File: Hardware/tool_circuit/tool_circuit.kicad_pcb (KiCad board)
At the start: 2 copper layers, 65 x 56.7 mm, 31 parts, among them J1 EJ503A, J2 Conn_01x03_Female, J3 Conn_01x08_Female, J4 GPIO_CONNECTOR, SW1 1825255-1, U1 LM2576D2TR4-5G

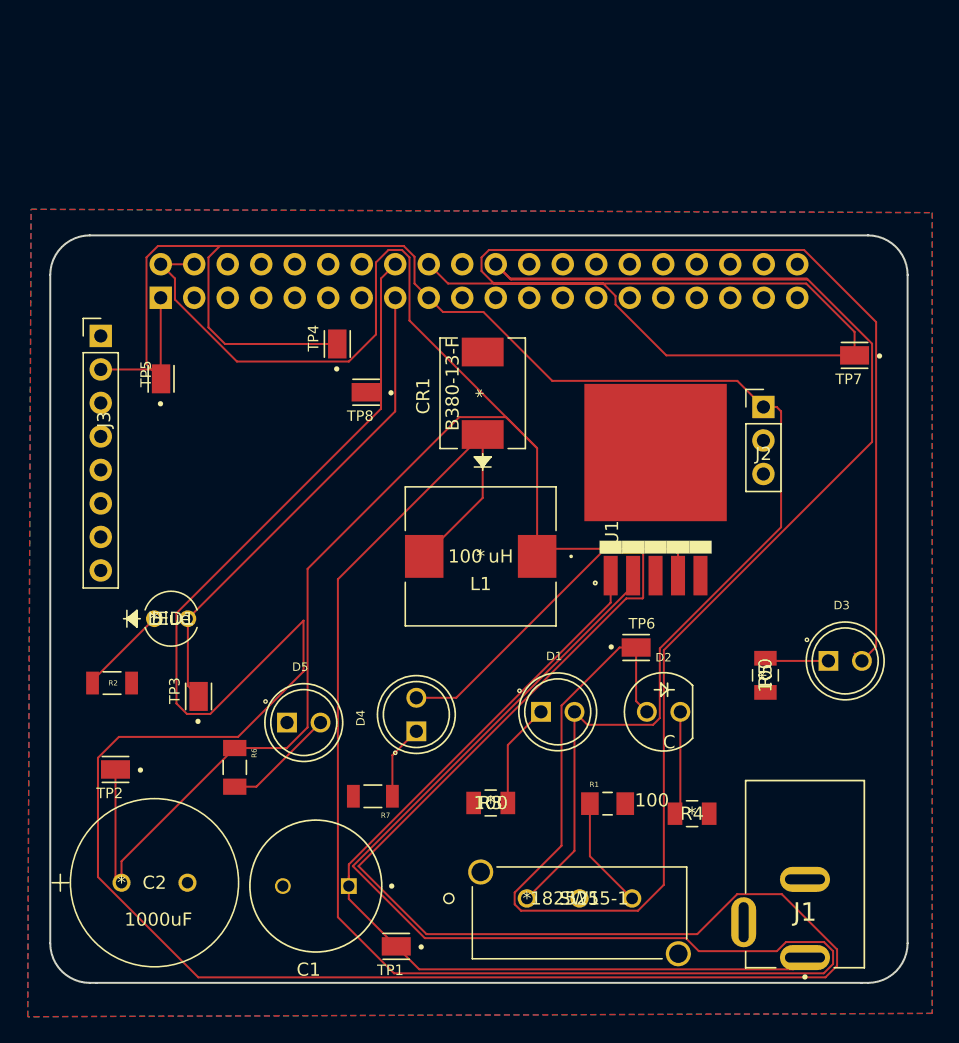
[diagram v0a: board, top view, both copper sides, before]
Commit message: pcb revisions
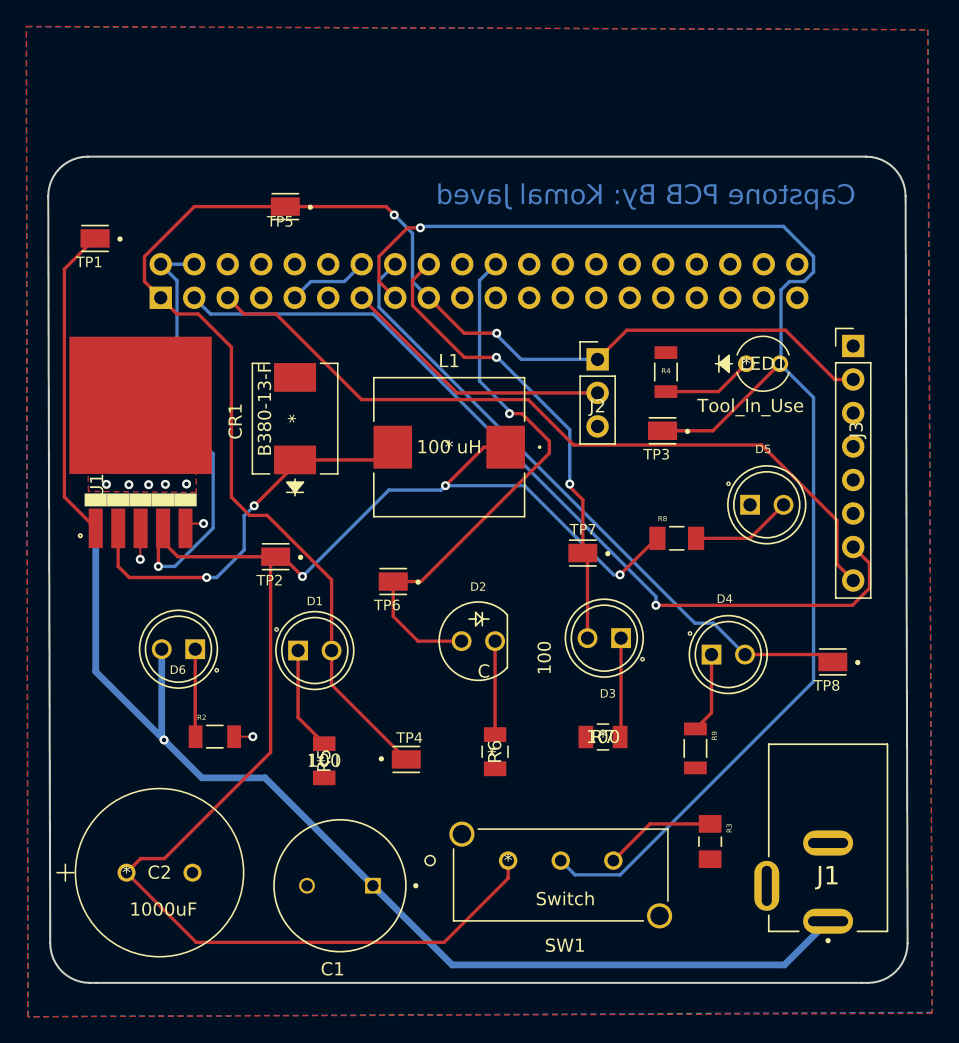
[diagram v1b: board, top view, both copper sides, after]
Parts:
- removed R1: 10k, RNCP1206FTD10K0:RESC3115X60N
- added D6: 12V, WP7113GD:LED_WP7113GD, F.Cu at (109.6, 79.7)
- added R8: 220, RMCF1206JT220R:RESC3216X70N, F.Cu at (147.4, 71.3)
- added R9: 130, AC1206FR-07130RL:RESC3116X65N, F.Cu at (148.8, 87.2)
- D1: value Green -> 3.3V
- D2: value Red -> Disable
- D3: value Green -> Enable
- D4: value Yellow -> Data_Transfer
- D5: value Green -> 5V
- J2: value Conn_01x03_Female -> Temp_Sense
- J3: value Conn_01x08_Female -> Accel.
- LED1: value Blue -> Tool_In_Use
- R2: value 42.2 -> 820; footprint RC1206FR-0742R2L:RESC3116X65N -> CRGCQ1206F820R:RESC3115X65N
- R3: value 100 -> 10k; footprint footprints:RNCP1206FTD100R -> RNCP1206FTD10K0:RESC3115X60N
- R4: value 100 -> 42.2; footprint footprints:RNCP1206FTD100R -> RC1206FR-0742R2L:RESC3116X65N
- R6: value 220 -> 100; footprint RMCF1206JT220R:RESC3216X70N -> footprints:RNCP1206FTD100R
- R7: value 130 -> 100; footprint AC1206FR-07130RL:RESC3116X65N -> footprints:RNCP1206FTD100R
- SW1: value 1825255-1 -> Switch
- TP1: value S2751-46R -> Vin
- TP2: value S2751-46R -> 5V_Reg_Vout
- TP3: value S2751-46R -> Tool_In_Use
- TP4: value S2751-46R -> 3.3V
- TP5: value S2751-46R -> GPIO1
- TP6: value S2751-46R -> Disable
- TP7: value S2751-46R -> Enable_LED
- TP8: value S2751-46R -> Data_Transfer
- moved TP1 58.3 mm to (103.3, 48.5)
- moved J3 57.1 mm to (160.8, 56.7)
- moved LED1 48.9 mm to (152.7, 58.0)
- moved TP8 40.9 mm to (159.2, 80.6)
- moved TP3 40.5 mm to (146.3, 63.1), turned to 180 degrees
- moved U1 39.2 mm to (106.7, 66.0)
- moved D5 38.8 mm to (154.2, 68.7)
- moved R5 34.1 mm to (120.7, 88.1)
- moved R4 33.5 mm to (146.6, 58.6), turned to 90 degrees
- moved TP4 31.9 mm to (126.9, 88.0), turned to 0 degrees
- moved TP7 25.5 mm to (140.3, 72.4)
- moved D4 24.1 mm to (151.3, 80.1), turned to 0 degrees
- moved TP2 20.2 mm to (117.0, 72.6)
- moved R6 19.8 mm to (133.6, 87.4)
- moved TP6 19.1 mm to (125.9, 74.5), turned to 180 degrees
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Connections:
- J2 pad 2: /Temp_Sense/GPIO27 -> GPIO27_GEN2
- J3 pad 7: /Accelerometer.sch/GPIO2 -> GPIO2_SDA1
- J3 pad 8: /Accelerometer.sch/GPIO3 -> GPIO3_SCL1
- J4 pad 13: /raspberrypi_header.sch/GPIO27 -> GPIO27_GEN2
- J4 pad 15: /raspberrypi_header.sch/GPIO22_GEN3 -> GPIO22_GEN3
- J4 pad 3: /raspberrypi_header.sch/GPIO2 -> GPIO2_SDA1
- J4 pad 5: /raspberrypi_header.sch/GPIO3 -> GPIO3_SCL1
- LED1 pad 2: /raspberrypi_header.sch/GPIO22_GEN3 -> GPIO22_GEN3
- R2 pad 1: Net-(LED1-Pad1) -> Net-(D6-PadC)
- R3 pad 1: Net-(D1-PadC) -> Net-(R3-Pad1)
- R4 pad 1: Net-(D2-Pad1) -> Net-(LED1-Pad1)
- R5 pad 1: Net-(D3-PadC) -> Net-(D1-PadC)
- R6 pad 1: +5V -> Net-(D2-Pad1)
- R6 pad 2: Net-(D5-PadA) -> GND
- R7 pad 1: Net-(D4-PadC) -> Net-(D3-PadC)
- SW1 pad 1: +3V3 -> +5V
- SW1 pad 2: /Time_of_Use/GPIO22 -> GPIO22_GEN3
- SW1 pad 3: Net-(R1-Pad1) -> Net-(R3-Pad1)
- TP3 pad 1: /raspberrypi_header.sch/GPIO22_GEN3 -> GPIO22_GEN3
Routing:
- net /raspberrypi_header.sch/Data_Transfer: track 241.6 -> 49.3 mm
- net Net-(CR1-Pad1): track 163.3 -> 29.9 mm, vias 0 -> 2
- net GPIO22_GEN3: track 0.00 -> 110.1 mm, vias 0 -> 1
- net /raspberrypi_header.sch/Disable_LED: track 144.2 -> 42.0 mm, vias 0 -> 1
- net /raspberrypi_header.sch/Enable_LED: track 127.9 -> 35.8 mm, vias 0 -> 2
- net GPIO2_SDA1: track 0.00 -> 65.4 mm, vias 0 -> 1
- net GPIO3_SCL1: track 0.00 -> 58.3 mm
- net +3V3: track 156.1 -> 112.9 mm, vias 0 -> 2
- net +12V: track 70.7 -> 107.9 mm, vias 0 -> 1
- net /raspberrypi_header.sch/GPIO22_GEN3: track 37.1 -> 0.00 mm
- net GPIO27_GEN2: track 0.00 -> 20.9 mm
- net +5V: track 136.0 -> 148.9 mm, vias 0 -> 4
- net GND: track 0.00 -> 11.4 mm, vias 0 -> 8
- net Net-(R1-Pad1): track 8.51 -> 0.00 mm
- net Net-(R3-Pad1): track 0.00 -> 8.49 mm
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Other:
- board size 65 x 56.7 mm -> 65.2 x 62.6 mm
- net class Default: clearance 0.1524 -> 0.254; trace_width 0.1524 -> 0.254
- rule trace_clearance: 0.1524 -> 0.254
- rule trace_min: 0.1524 -> 0.254
- board text added: "Capstone PCB By: Komal Javed"
